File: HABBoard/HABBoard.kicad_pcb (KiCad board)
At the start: 4 copper layers, 100 x 100 mm, 213 parts, among them J1 USB_C_MCU, J10 RFShield_TwoPieces, J2 USB_C_GNSS, J3 MEM2067-02-180-00-A_REVB, J4 GPS In, J5 GNSS_UART, J6 DEBUG, J7 VHF Out, J8 UHF Out, J9 RFShield_TwoPieces, Q1 SSM6N7002KFU, Q2 SSM6N7002KFU, Q3 SSM6N7002KFU, Q4 PMN16XNE, SW1 RESET, SW2 BOOT, SW3 USER_BUTTON, SW4 Power, U1 TC2015-3.3VxCTTR, U10 SX1276, U11 SX1276, U12 MP5016GQH-Z, U13 PE42421, U14 ISL91127IR, U15 TPS2116DRLR, U16 INA219BxD, U2 W25Q128JVS, U3 NEO-M9N-00B, U4 AP2138N-2.5, U5 RP2040, U6 BME680, U7 TXS0104E, U8 ICM-20948, U9 AP2138N-1.8, Y1 ECS-TXO-25CSMV-320-BM-TR, Y2 ECS-TXO-25CSMV-320-BM-TR, Y3 12.000MHz

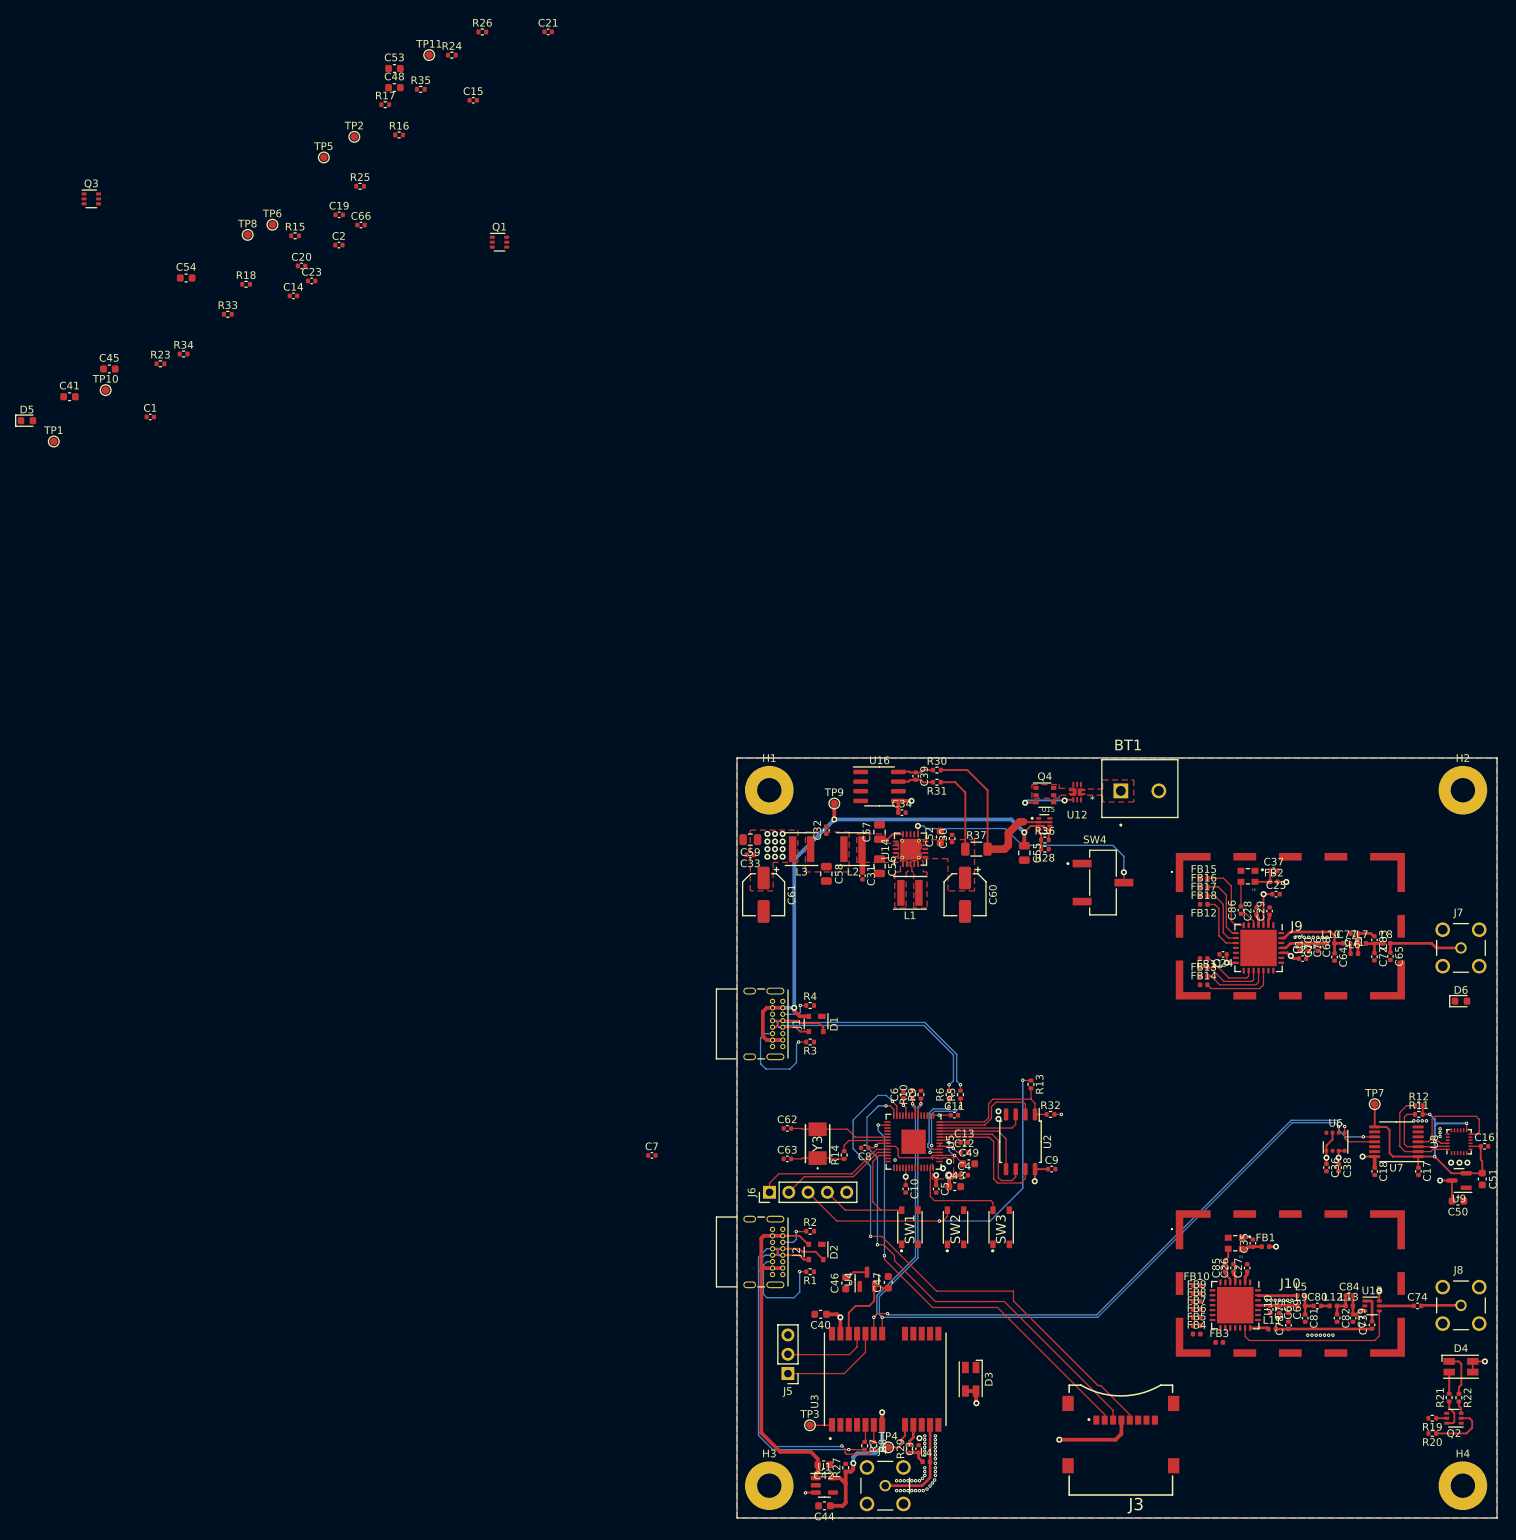
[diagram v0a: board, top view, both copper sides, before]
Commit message: Even more layout
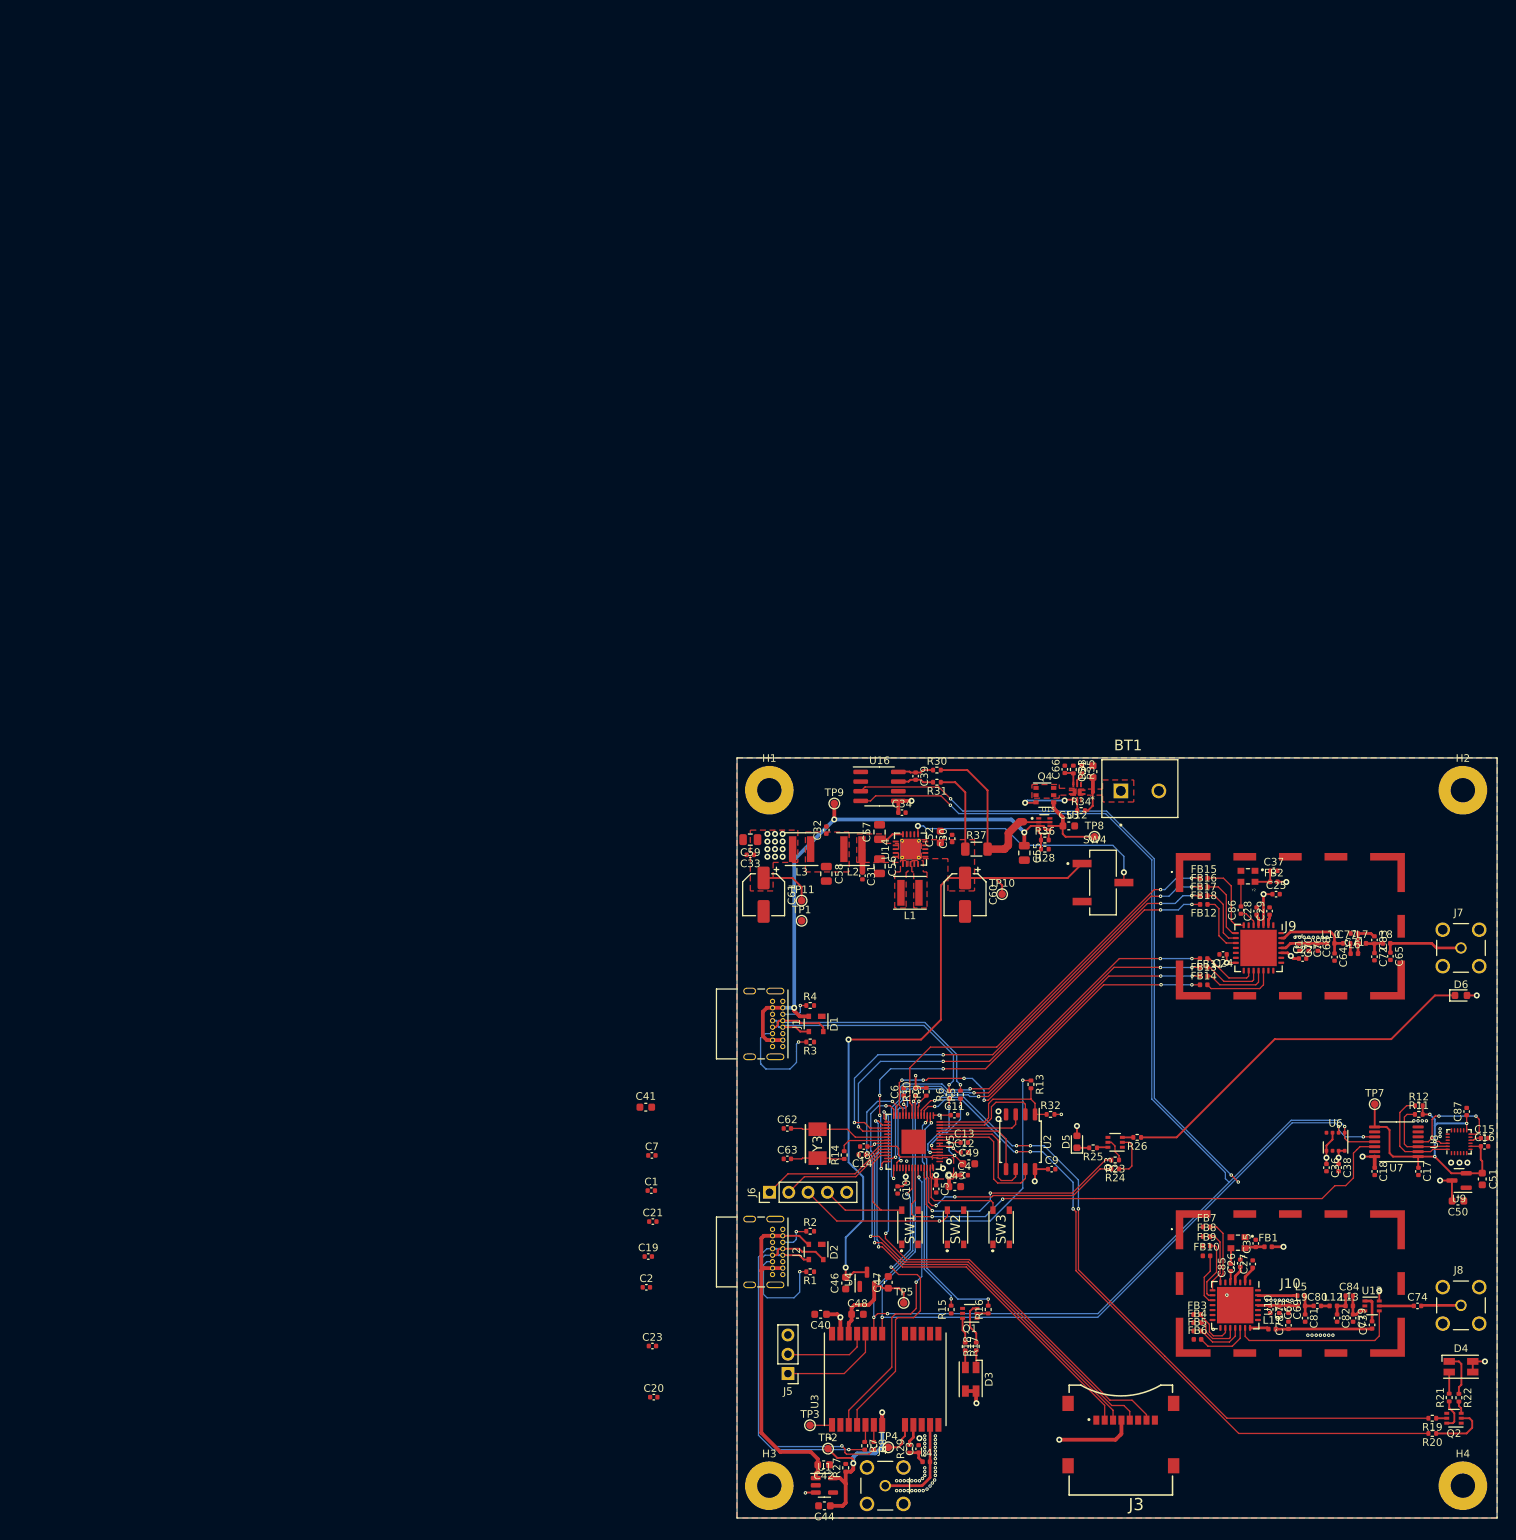
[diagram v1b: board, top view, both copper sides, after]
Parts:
- removed C45: 1u, Capacitor_SMD:C_0603_1608Metric
- removed TP6: VCORE, TestPoint:TestPoint_Pad_D1.0mm
- added C87: 0.1u, Capacitor_SMD:C_0402_1005Metric, F.Cu at (123.8, 71.5)
- moved C15 190.6 mm to (126.1, 75.0)
- moved TP2 183.5 mm to (39.7, 115.9)
- moved Q3 183.2 mm to (77.5, 75.6), turned to 180 degrees
- moved R17 180.3 mm to (57.8, 102.4), turned to -90 degrees
- moved R16 172.9 mm to (60.8, 97.6), turned to 90 degrees
- moved C48 172.5 mm to (43.6, 98.2)
- moved R24 170.6 mm to (77.5, 79.1), turned to 180 degrees
- moved R18 169.6 mm to (59.2, 102.4), turned to 90 degrees
- moved R26 169.0 mm to (80.4, 74.9), turned to 180 degrees
- moved TP5 168.9 mm to (49.7, 96.7)
- moved D5 167.6 mm to (72.5, 75.5), turned to 90 degrees
- moved R15 165.5 mm to (55.9, 97.6), turned to 90 degrees
- moved R23 163.6 mm to (77.5, 77.9), turned to 180 degrees
- moved R25 159.1 mm to (74.6, 76.3), turned to 180 degrees
- moved C21 157.1 mm to (16.7, 86.0)
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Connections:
- J10 pad 10: (no net) -> GND
- J10 pad 11: (no net) -> GND
- J10 pad 12: (no net) -> GND
- J10 pad 13: (no net) -> GND
- J10 pad 14: (no net) -> GND
- J10 pad 15: (no net) -> GND
- J10 pad 16: (no net) -> GND
- J10 pad 2: (no net) -> GND
- J10 pad 3: (no net) -> GND
- J10 pad 4: (no net) -> GND
- J10 pad 5: (no net) -> GND
- J10 pad 6: (no net) -> GND
- J10 pad 7: (no net) -> GND
- J10 pad 8: (no net) -> GND
- J10 pad 9: (no net) -> GND
- J9 pad 10: (no net) -> GND
- J9 pad 11: (no net) -> GND
- J9 pad 12: (no net) -> GND
- J9 pad 13: (no net) -> GND
- J9 pad 14: (no net) -> GND
- J9 pad 15: (no net) -> GND
- J9 pad 16: (no net) -> GND
- J9 pad 2: (no net) -> GND
- J9 pad 3: (no net) -> GND
- J9 pad 4: (no net) -> GND
- J9 pad 5: (no net) -> GND
- J9 pad 6: (no net) -> GND
- J9 pad 7: (no net) -> GND
- J9 pad 8: (no net) -> GND
- J9 pad 9: (no net) -> GND
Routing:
- net /UHF_SRED: track 0.00 -> 92.6 mm, vias 0 -> 4
- net /UHF_SGRN: track 0.00 -> 92.4 mm, vias 0 -> 4
- net /BME_SDA: track 112.3 -> 203.4 mm, vias 4 -> 7
- net +SYS: track 14.3 -> 104.5 mm, vias 0 -> 2
- net /BME_SCL: track 113.9 -> 203.0 mm, vias 4 -> 5
- net /IMU_INT: track 0.00 -> 73.0 mm, vias 0 -> 2
- net /VHF_DIO0: track 0.00 -> 66.4 mm, vias 0 -> 4
- net /VHF_DIO2: track 0.00 -> 65.0 mm, vias 0 -> 6
- net /VHF_DIO1: track 0.00 -> 64.9 mm, vias 0 -> 4
- net /SD_MISO: track 0.00 -> 63.3 mm, vias 0 -> 2
- net /RF_SCK: track 0.00 -> 61.1 mm, vias 0 -> 4
- net /RF_MOSI: track 0.00 -> 57.7 mm, vias 0 -> 4
- net /RF_MISO: track 0.00 -> 57.1 mm, vias 0 -> 4
- net /VHF_RESET: track 0.00 -> 54.9 mm, vias 0 -> 2
- net /VHF_NSS: track 0.00 -> 52.6 mm, vias 0 -> 6
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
